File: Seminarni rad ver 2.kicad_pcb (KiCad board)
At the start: 2 copper layers, 116.8 x 91.4 mm, 35 parts, among them J1 Screw_Terminal_01x02 (Izlaz), J2 Screw_Terminal_01x02(power), J3 Screw_Terminal_01x02(ulaz), Q1 IRLZ44N, Q4 2N7000, SW1 SW_Nidec_CAS-120A1, U2 NE555P, U3 DL1416, U4 ATtiny3217-M, U5 INA260, X7RDielectric2 100n

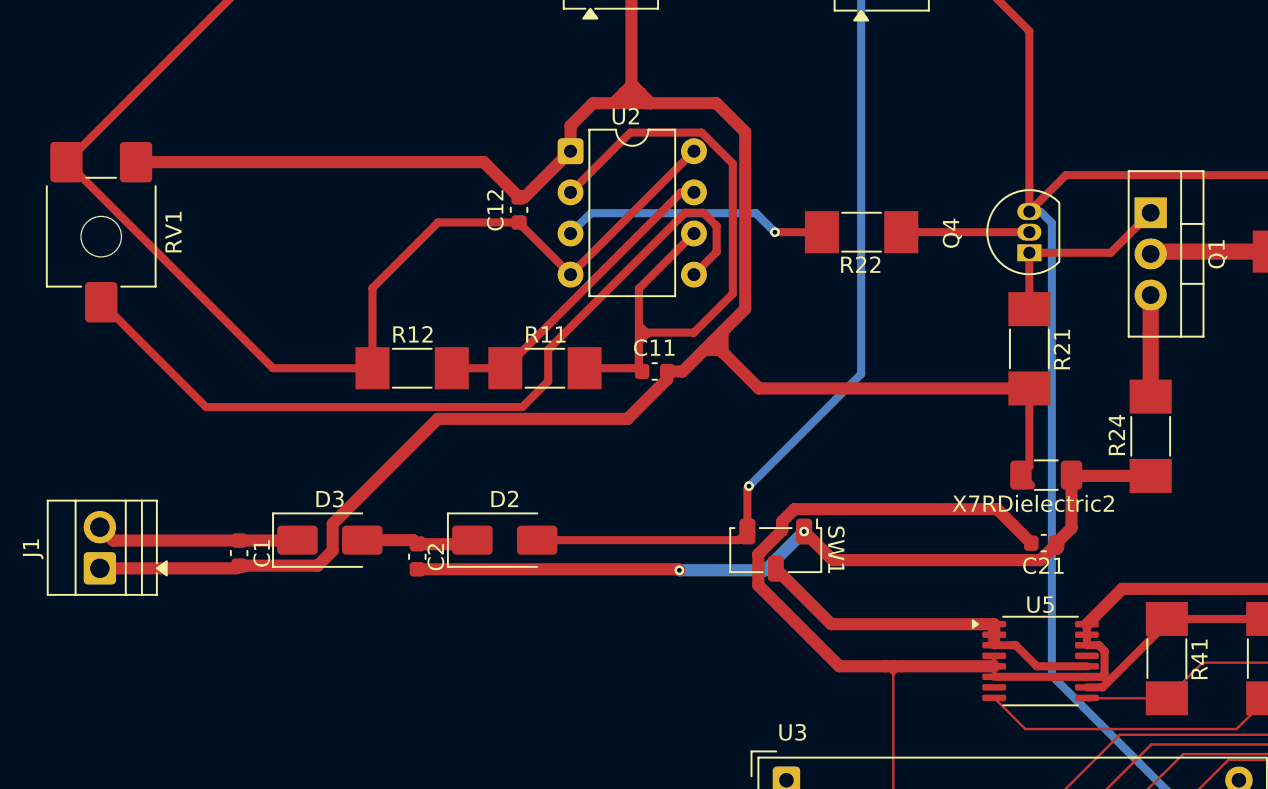
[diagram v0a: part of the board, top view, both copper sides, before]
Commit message: chande
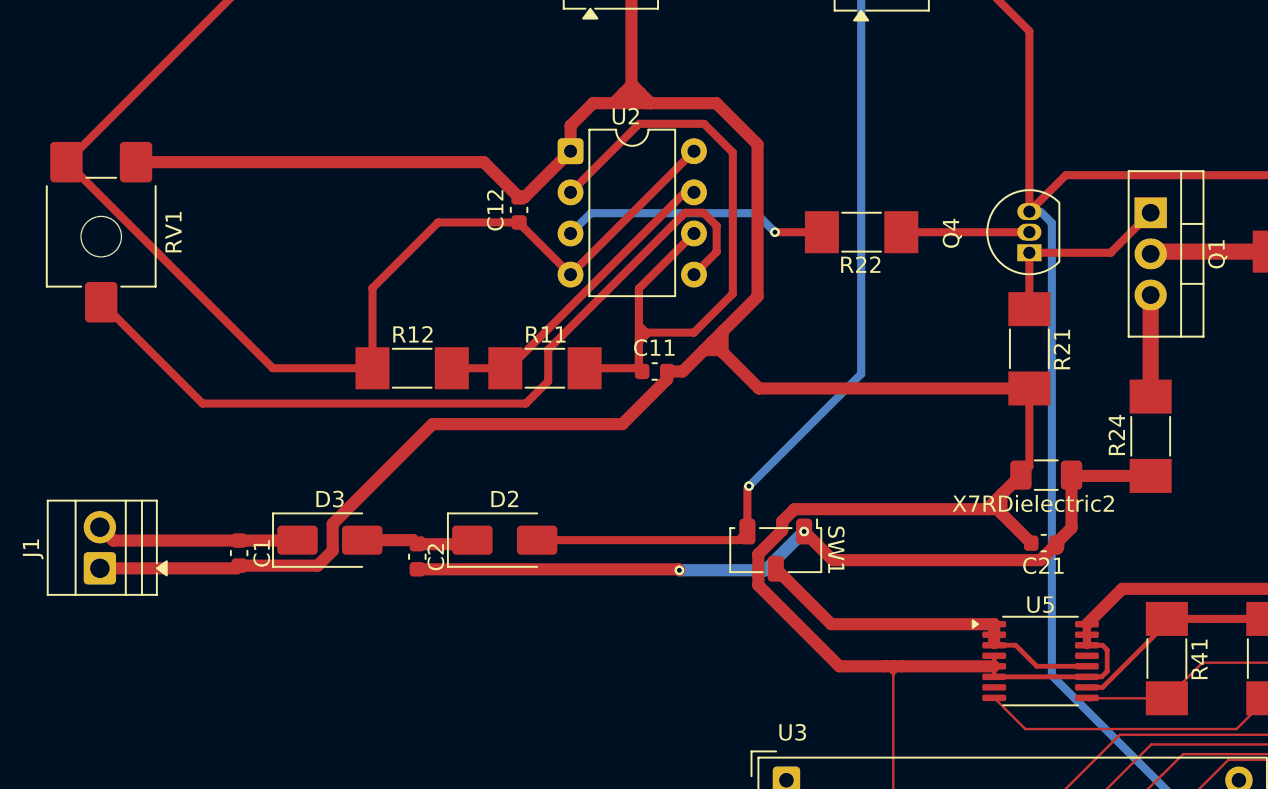
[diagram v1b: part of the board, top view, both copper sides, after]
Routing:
- net GND: track 338.3 -> 342.6 mm
- net Net-(U2-THR): track 44.9 -> 45.8 mm
